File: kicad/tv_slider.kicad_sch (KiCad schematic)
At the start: 10 parts, among them J1 MC 1,5/2-G-3.81, J2 MC 1,5/6-G-3.81, J3 MC 1,5/4-G-3.81, J4 MC 1,5/3-G-3.81, J5 MC 1,5/3-G-3.81, J6 MC 1,5/3-G-3.81, J7 MC 1,5/3-G-3.81

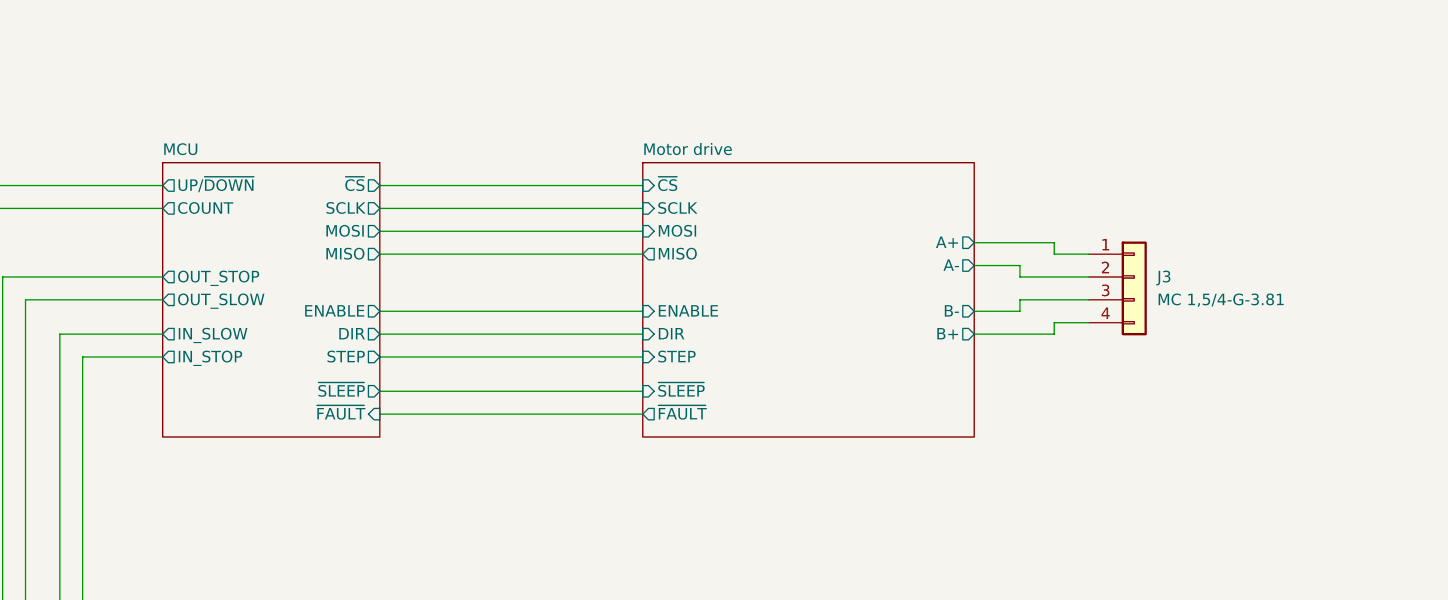
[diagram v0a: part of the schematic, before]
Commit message: Reviewed the ESP32-C6-DEVKIT GPIO's. Some of them have a dual function and are better left untouched.
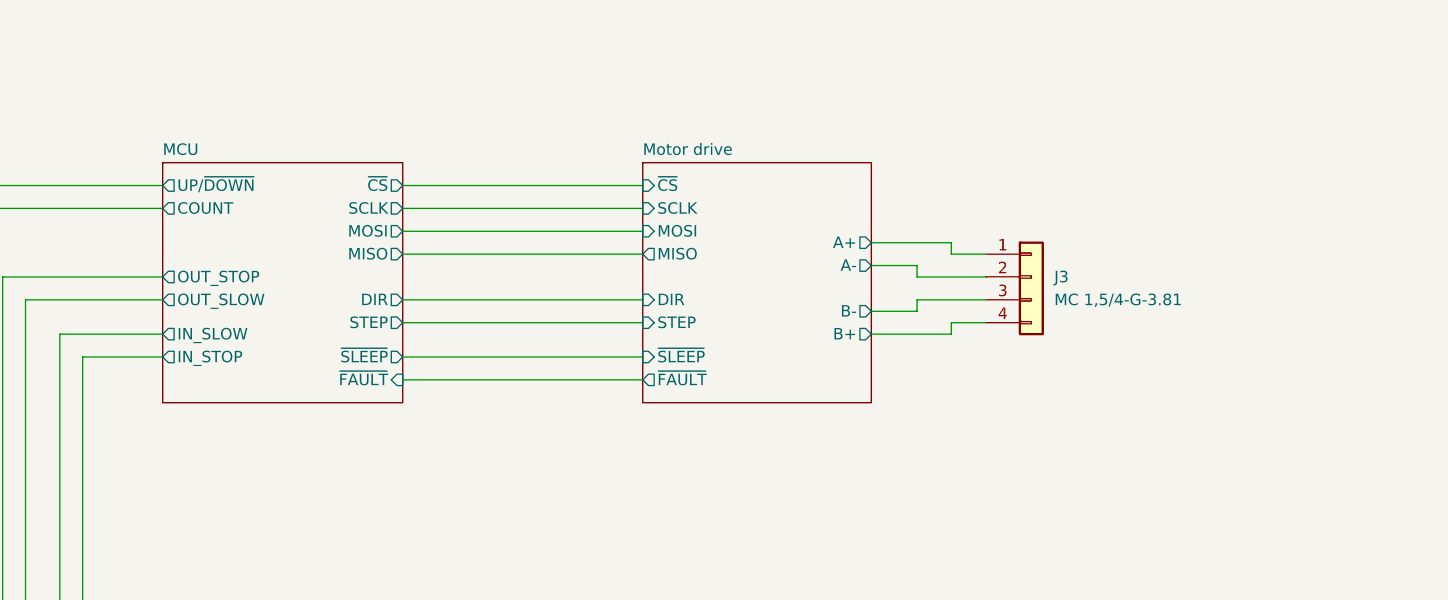
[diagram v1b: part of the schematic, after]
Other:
- sheet MCU ports: added none; removed ENABLE
- sheet Motor drive ports: added none; removed ENABLE
- moved on the sheet: J3
